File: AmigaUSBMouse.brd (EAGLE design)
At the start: 64.2 x 32.7 mm, 14 parts

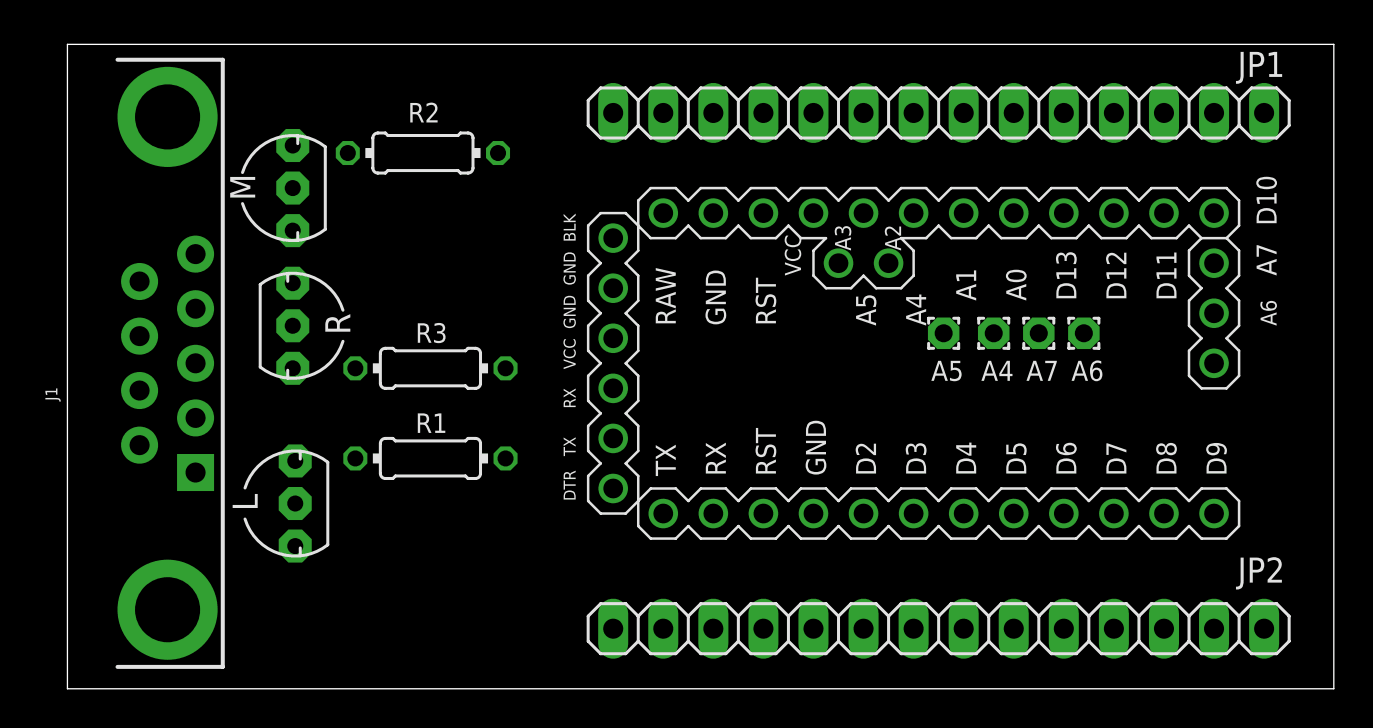
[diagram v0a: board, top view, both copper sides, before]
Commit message: Initial
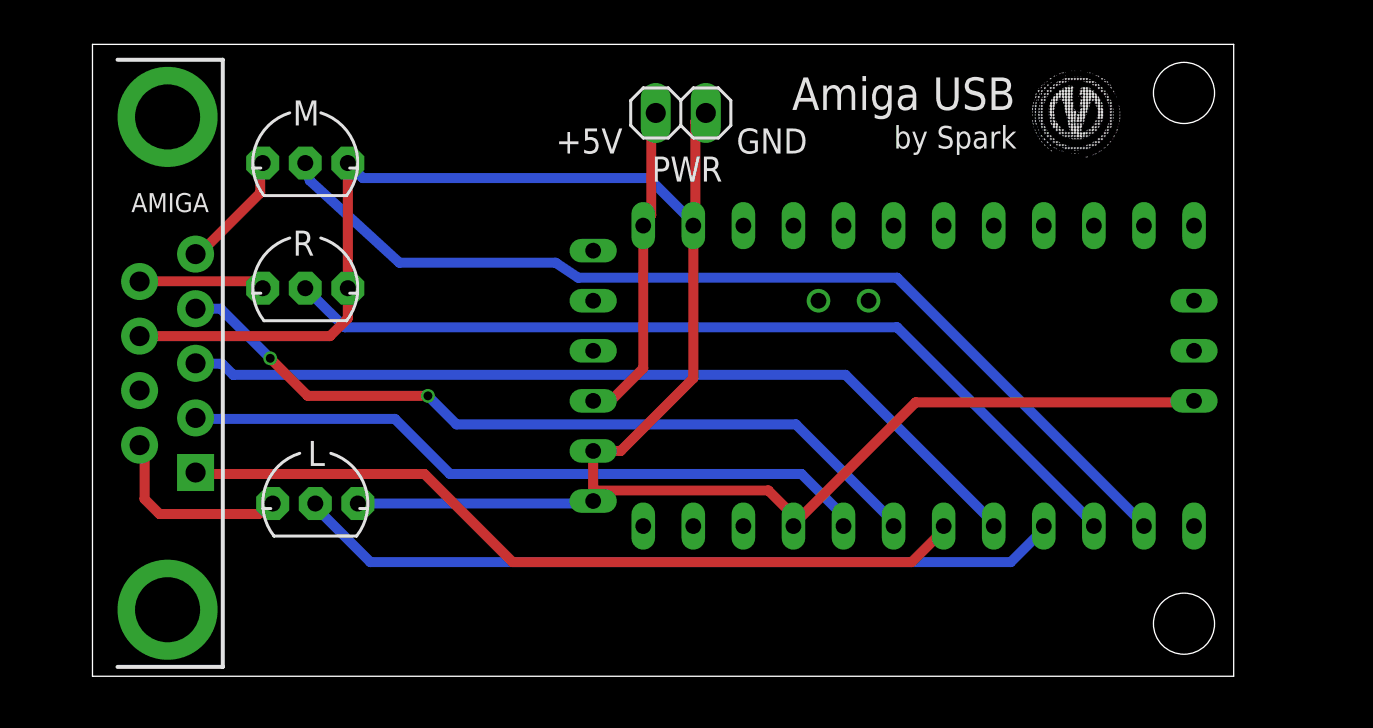
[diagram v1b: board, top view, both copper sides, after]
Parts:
- removed A4, A5, A6, A7: WIREPAD2,15/1,0, wirepad:1,6/0,9
- removed ARDUINO1: (no value), arduinopromini:ARDUINO_PRO_MINI
- removed JP1, JP2: (no value), pinhead:1X14
- removed R1, R2, R3: (no value), rcl:0204/7
- added PWR: (no value), pinhead:1X02
- added U$1: ABK-PRO-MINI, Arduino-clone:ABK-PRO-MINI
- L, M, R: value FQN1N50CI -> BS108
- moved R 2.01 mm to (12.1, 20.3), turned to 0 degrees
- moved M 1.42 mm to (12.1, 26.7), turned to 0 degrees
- moved L 1.02 mm to (12.6, 9.40), turned to 0 degrees
- renumbered J1 to AMIGA
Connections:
- removed net A4: A4.1, ARDUINO1.A4
- removed net A5: A5.1, ARDUINO1.A5
- removed net H: AMIGA.2
- removed net HQ: AMIGA.4
- removed net N$1: L.3, R1.1
- removed net N$2: M.3, R2.1
- removed net N$3: R.3, R3.1
- removed net RX: ARDUINO1.RX, ARDUINO1.RX@1, JP2.3
- removed net TX: ARDUINO1.TX, ARDUINO1.TX@1, JP2.2
- removed net V: AMIGA.1
- removed net VQ: AMIGA.3
- new net RST1: U$1.RST1
- new net RX1: U$1.RX1
- new net RX2: U$1.RX1-1
- new net TX1: U$1.TX0
- new net TX2: U$1.TX0-1
- net A0: now also U$1.A0; no longer ARDUINO1.A0, JP1.9
- net A1: now also U$1.A1; no longer ARDUINO1.A1, JP1.8
- net A2: now also U$1.A2; no longer ARDUINO1.A2, JP1.7
- net A3: now also U$1.A3; no longer ARDUINO1.A3, JP1.6
- net A6: now also U$1.A6; no longer A6.1, ARDUINO1.A6
- net A7: now also U$1.A7; no longer A7.1, ARDUINO1.A7
- net D10: now also U$1.D10; no longer ARDUINO1.D10, JP1.13
- net D11: now also U$1.D11; no longer ARDUINO1.D11, JP1.12
- net D12: now also U$1.D12; no longer ARDUINO1.D12, JP1.11
- net D13: now also U$1.D13; no longer ARDUINO1.D13, JP1.10
- net D9: now also U$1.D9; no longer ARDUINO1.D9, JP2.13
- net DTR: now also U$1.DTR; no longer ARDUINO1.DTR, JP2.1
- net GND: now also L.3, M.3, PWR.1, R.3, U$1.GND, U$1.GND1, U$1.GND2, U$1.GND3, U$1.GND4; no longer ARDUINO1.GND, ARDUINO1.GND@1, ARDUINO1.GND@2, ARDUINO1.GND@3, JP1.14, JP1.3, JP1.4, JP2.14, JP2.5, R1.2, R2.2, R3.2
- net MOUSE_LEFT: now also U$1.D6; no longer ARDUINO1.D6, JP2.10
- net MOUSE_MIDDLE: now also U$1.D8; no longer ARDUINO1.D8, JP2.12
- net MOUSE_RIGHT: now also U$1.D7; no longer ARDUINO1.D7, JP2.11
- net RAW: now also PWR.2, U$1.RAW, U$1.VCC1; no longer AMIGA.7, ARDUINO1.RAW, JP1.1, JP1.2
- net RST: now also U$1.RST; no longer ARDUINO1.RST, ARDUINO1.RST@1, JP2.4
- net VCC: now also U$1.VCC; no longer ARDUINO1.VCC, ARDUINO1.VCC@1, JP1.5
- net X1_VQ: now also AMIGA.3, U$1.D5; no longer ARDUINO1.D5, JP2.9
- net X2_V: now also AMIGA.1, U$1.D4; no longer ARDUINO1.D4, JP2.8
- net Y1_HQ: now also AMIGA.4, U$1.D3; no longer ARDUINO1.D3, JP2.7
- net Y2_H: now also AMIGA.2, U$1.D2; no longer ARDUINO1.D2, JP2.6
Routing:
- net GND: track 0.00 -> 108.0 mm
- net MOUSE_MIDDLE: track 0.00 -> 50.5 mm
- net MOUSE_RIGHT: track 0.00 -> 45.0 mm
- net X1_VQ: track 0.00 -> 44.1 mm
- net X2_V: track 0.00 -> 40.8 mm
- net Y1_HQ: track 0.00 -> 40.2 mm, vias 0 -> 2
- net MOUSE_LEFT: track 0.00 -> 39.2 mm
- net Y2_H: track 0.00 -> 35.4 mm
- net RAW: track 0.00 -> 16.4 mm
- net BTN_L: track 0.00 -> 9.92 mm
- net BTN_R: track 0.00 -> 6.43 mm
- net BTN_M: track 0.00 -> 6.13 mm
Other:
- board size 64.2 x 32.7 mm -> 57.9 x 32.1 mm
- board text added: "+5V"
- board text added: "Amiga USB"
- board text added: "Arduino Pro Mini & USB Mini Shield"
- board text added: "GND"
- board text added: "by Spark"
